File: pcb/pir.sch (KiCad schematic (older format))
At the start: 0 parts

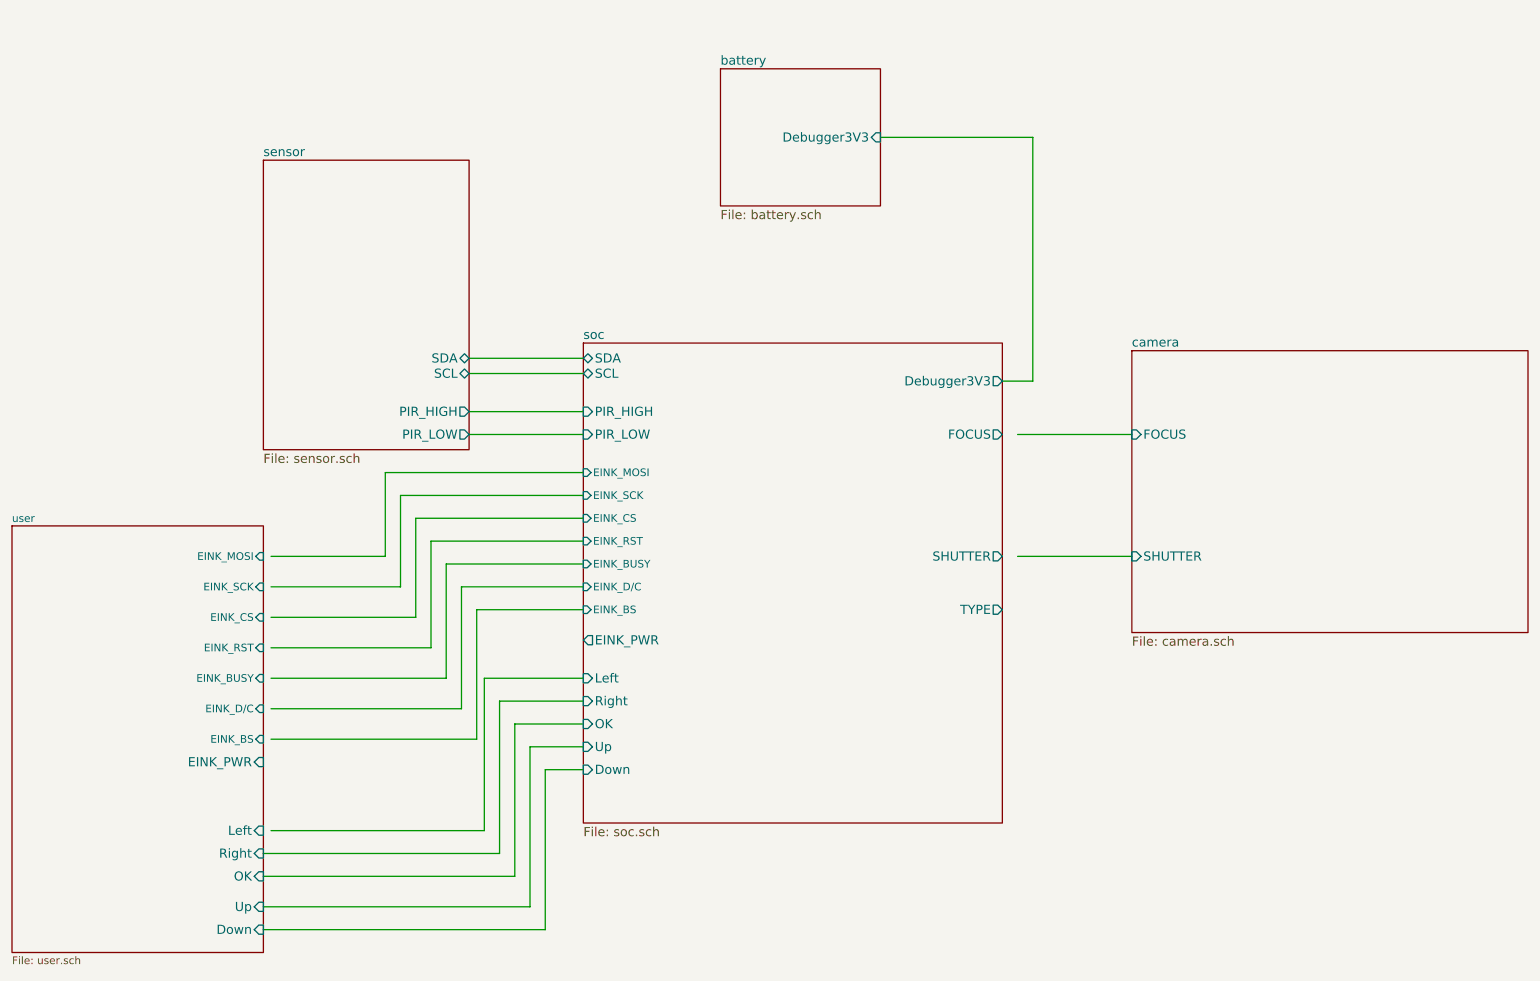
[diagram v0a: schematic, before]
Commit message: Reworked the front diagram
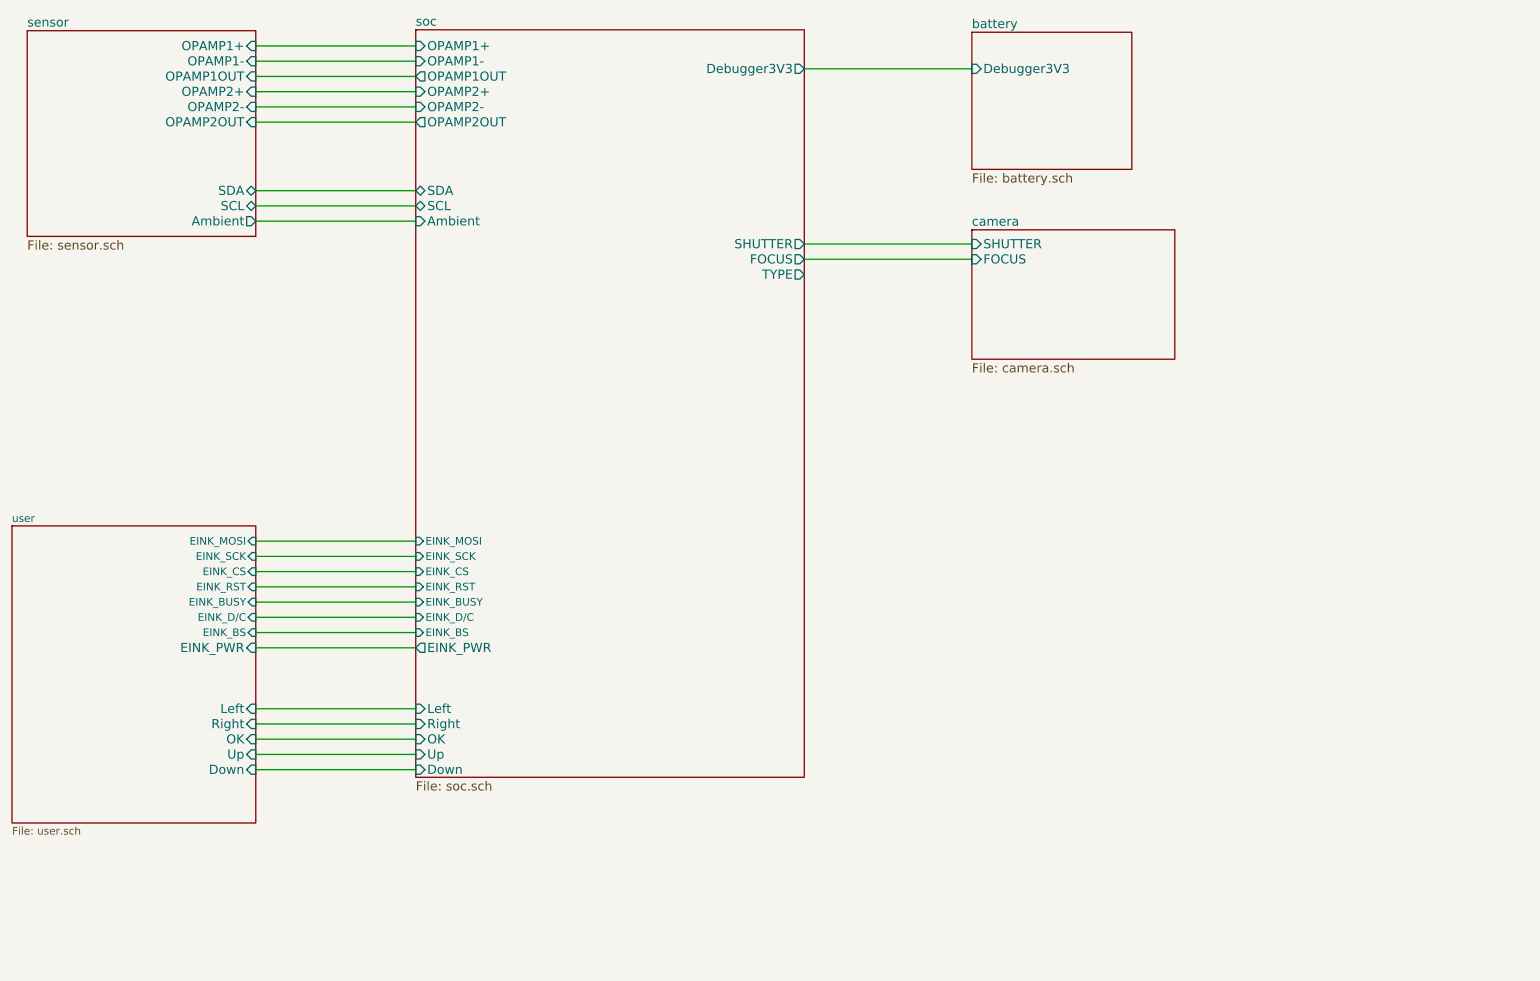
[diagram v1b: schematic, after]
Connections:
- wire segments 45 -> 25
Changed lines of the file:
@@
 LIBS:ab2_usb
 LIBS:ab2_xtal
-LIBS:pir-cache
 EELAYER 25 0
 EELAYER END
@@
 $EndDescr
 $Sheet
-S 2450 1750 1350 1900
+S 900  900  1500 1350
 U 5A768E85
 F0 "sensor" 60
 F1 "sensor.sch" 60
-F2 "PIR_HIGH" O R 3800 3400 60
-F3 "PIR_LOW" O R 3800 3550 60
-F4 "SDA" B R 3800 3050 60
-F5 "SCL" B R 3800 3150 60
+F2 "SDA" B R 2400 1950 60
+F3 "SCL" B R 2400 2050 60
+F4 "Ambient" O R 2400 2150 60
+F5 "OPAMP1+" I R 2400 1000 60
+F6 "OPAMP1-" I R 2400 1100 60
+F7 "OPAMP1OUT" I R 2400 1200 60
+F8 "OPAMP2-" I R 2400 1400 60
+F9 "OPAMP2+" I R 2400 1300 60
+F10 "OPAMP2OUT" I R 2400 1500 60
 $EndSheet
 $Sheet
-S 5450 1150 1050 900
+S 7100 910  1050 900
 U 5A769BAC
 F0 "battery" 60
 F1 "battery.sch" 60
-F2 "Debugger3V3" I R 6500 1600 60
+F2 "Debugger3V3" I L 7100 1150 60
 $EndSheet
 $Sheet
-S 4550 2950 2750 3150
+S 7100 2207 1332 849
+U 5A76C721
+F0 "camera" 60
+F1 "camera.sch" 60
+F2 "FOCUS" I L 7100 2400 60
+F3 "SHUTTER" I L 7100 2300 60
+$EndSheet
+$Sheet
+S 800  4150 1600 1950
+U 5A7EC53C
+F0 "user" 50
+F1 "user.sch" 50
+F2 "EINK_MOSI" I R 2400 4250 50
+F3 "EINK_SCK" I R 2400 4350 50
+F4 "EINK_CS" I R 2400 4450 50
+F5 "EINK_RST" I R 2400 4550 50
+F6 "EINK_BUSY" I R 2400 4650 50
+F7 "EINK_D/C" I R 2400 4750 50
+F8 "EINK_BS" I R 2400 4850 50
+F9 "EINK_PWR" I R 2400 4950 60
+F10 "Down" I R 2400 5750 60
+F11 "Right" I R 2400 5450 60
+F12 "OK" I R 2400 5550 60
+F13 "Up" I R 2400 5650 60
+F14 "Left" I R 2400 5350 60
+$EndSheet
+$Sheet
+S 3450 894  2550 4906
 U 5A76AF1D
 F0 "soc" 60
 F1 "soc.sch" 60
-F2 "PIR_HIGH" I L 4550 3400 60
-F3 "PIR_LOW" I L 4550 3550 60
-F4 "FOCUS" O R 7300 3550 60
-F5 "SHUTTER" O R 7300 4350 60
-F6 "Debugger3V3" O R 7300 3200 60
-F7 "EINK_SCK" I L 4550 3950 50
-F8 "EINK_MOSI" I L 4550 3800 50
-F9 "EINK_CS" I L 4550 4100 50
-F10 "EINK_RST" I L 4550 4250 50
-F11 "EINK_BUSY" I L 4550 4400 50
-F12 "EINK_D/C" I L 4550 4550 50
-F13 "EINK_BS" I L 4550 4700 50
-F14 "EINK_PWR" O L 4550 4900 60
-F15 "TYPE" O R 7300 4700 60
-F16 "SCL" B L 4550 3150 60
-F17 "SDA" B L 4550 3050 60
-F18 "Left" I L 4550 5150 60
-F19 "Right" I L 4550 5300 60
-F20 "Up" I L 4550 5600 60
-F21 "Down" I L 4550 5750 60
-F22 "OK" I L 4550 5450 60
+F2 "FOCUS" O R 6000 2400 60
+F3 "SHUTTER" O R 6000 2300 60
+F4 "Debugger3V3" O R 6000 1150 60
+F5 "EINK_SCK" I L 3450 4350 50
+F6 "EINK_MOSI" I L 3450 4250 50
+F7 "EINK_CS" I L 3450 4450 50
+F8 "EINK_RST" I L 3450 4550 50
+F9 "EINK_BUSY" I L 3450 4650 50
+F10 "EINK_D/C" I L 3450 4750 50
+F11 "EINK_BS" I L 3450 4850 50
+F12 "EINK_PWR" O L 3450 4950 60
+F13 "TYPE" O R 6000 2500 60
+F14 "SCL" B L 3450 2050 60
+F15 "SDA" B L 3450 1950 60
+F16 "Left" I L 3450 5350 60
+F17 "Right" I L 3450 5450 60
+F18 "Up" I L 3450 5650 60
+F19 "Down" I L 3450 5750 60
+F20 "OK" I L 3450 5550 60
+F21 "OPAMP1+" I L 3450 1000 60
+F22 "OPAMP1-" I L 3450 1100 60
+F23 "OPAMP1OUT" O L 3450 1200 60
+F24 "OPAMP2+" I L 3450 1300 60
+F25 "OPAMP2-" I L 3450 1400 60
+F26 "OPAMP2OUT" O L 3450 1500 60
+F27 "Ambient" I L 3450 2150 60
 $EndSheet
 Wire Wire Line
-	3800 3550 4550 3550
-$Sheet
-S 8150 3000 2600 1850
-U 5A76C721
-F0 "camera" 60
-F1 "camera.sch" 60
-F2 "FOCUS" I L 8150 3550 60
-F3 "SHUTTER" I L 8150 4350 60
-$EndSheet
+	3450 1950 2400 1950
 Wire Wire Line
-	7400 3550 8150 3550
+	2400 2050 3450 2050
 Wire Wire Line
-	7400 4350 8150 4350
-$Sheet
-S 800  4150 1650 2800
-U 5A7EC53C
-F0 "user" 50
-F1 "user.sch" 50
-F2 "EINK_MOSI" I R 2450 4350 50
-F3 "EINK_SCK" I R 2450 4550 50
-F4 "EINK_CS" I R 2450 4750 50
-F5 "EINK_RST" I R 2450 4950 50
-F6 "EINK_BUSY" I R 2450 5150 50
-F7 "EINK_D/C" I R 2450 5350 50
-F8 "EINK_BS" I R 2450 5550 50
-F9 "EINK_PWR" I R 2450 5700 60
-F10 "Down" I R 2450 6800 60
-F11 "Right" I R 2450 6300 60
-F12 "OK" I R 2450 6450 60
-F13 "Up" I R 2450 6650 60
-F14 "Left" I R 2450 6150 60
-$EndSheet
+	2400 1000 3450 1000
 Wire Wire Line
-	3800 3400 4550 3400
+	2400 1100 3450 1100
 Wire Wire Line
-	2500 4350 3250 4350
+	2400 1200 3450 1200
 Wire Wire Line
-	3250 4350 3250 3800
+	2400 1300 3450 1300
 Wire Wire Line
-	3250 3800 4550 3800
+	3450 1400 2400 1400
 Wire Wire Line
-	2500 4550 3350 4550
+	2400 1500 3450 1500
 Wire Wire Line
-	3350 4550 3350 3950
+	2400 2150 3450 2150
 Wire Wire Line
-	3350 3950 4550 3950
+	2400 4250 3450 4250
 Wire Wire Line
-	2500 4750 3450 4750
+	2400 4350 3450 4350
 Wire Wire Line
-	3450 4750 3450 4100
+	2400 4450 3450 4450
 Wire Wire Line
-	3450 4100 4550 4100
+	2400 4550 3450 4550
 Wire Wire Line
-	2500 4950 3550 4950
+	2400 4650 3450 4650
 Wire Wire Line
-	3550 4950 3550 4250
+	2400 4750 3450 4750
 Wire Wire Line
-	3550 4250 4550 4250
+	2400 4850 3450 4850
 Wire Wire Line
-	2500 5150 3650 5150
+	2400 4950 3450 4950
 Wire Wire Line
-	3650 5150 3650 4400
+	2400 5350 3450 5350
 Wire Wire Line
-	3650 4400 4550 4400
+	2400 5450 3450 5450
 Wire Wire Line
-	2500 5350 3750 5350
+	2400 5550 3450 5550
 Wire Wire Line
-	3750 5350 3750 4550
+	2400 5650 3450 5650
 Wire Wire Line
-	3750 4550 4550 4550
+	2400 5750 3450 5750
 Wire Wire Line
-	3850 5550 3850 4700
+	6000 1150 7100 1150
 Wire Wire Line
-	3850 4700 4550 4700
+	7100 2300 6000 2300
 Wire Wire Line
-	2500 5550 3850 5550
-Wire Wire Line
-	6500 1600 7500 1600
-Wire Wire Line
-	7500 1600 7500 3200
-Wire Wire Line
-	7500 3200 7300 3200
-Wire Wire Line
-	3800 3150 4550 3150
-Wire Wire Line
-	4550 3050 3800 3050
-Wire Wire Line
-	2500 6150 3900 6150
-Wire Wire Line
-	3900 6150 3900 5150
-Wire Wire Line
-	3900 5150 4550 5150
-Wire Wire Line
-	2450 6300 4000 6300
-Wire Wire Line
-	4000 6300 4000 5300
-Wire Wire Line
-	4000 5300 4550 5300
-Wire Wire Line
-	2450 6450 4100 6450
-Wire Wire Line
-	4100 6450 4100 5450
-Wire Wire Line
-	4100 5450 4550 5450
-Wire Wire Line
-	2450 6650 4200 6650
-Wire Wire Line
-	4200 6650 4200 5600
-Wire Wire Line
-	4200 5600 4550 5600
-Wire Wire Line
-	2450 6800 4300 6800
-Wire Wire Line
-	4300 6800 4300 5750
-Wire Wire Line
-	4300 5750 4550 5750
+	6000 2400 7100 2400
 $EndSCHEMATC
